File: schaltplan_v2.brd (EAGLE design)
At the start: 101 x 80 mm, 42 parts, among them T1 2N3565, T2 2N3565, T3 2N3565, T4 2N3565, T5 2N3565, T6 2N3565, T7 2N3565, T8 2N3565

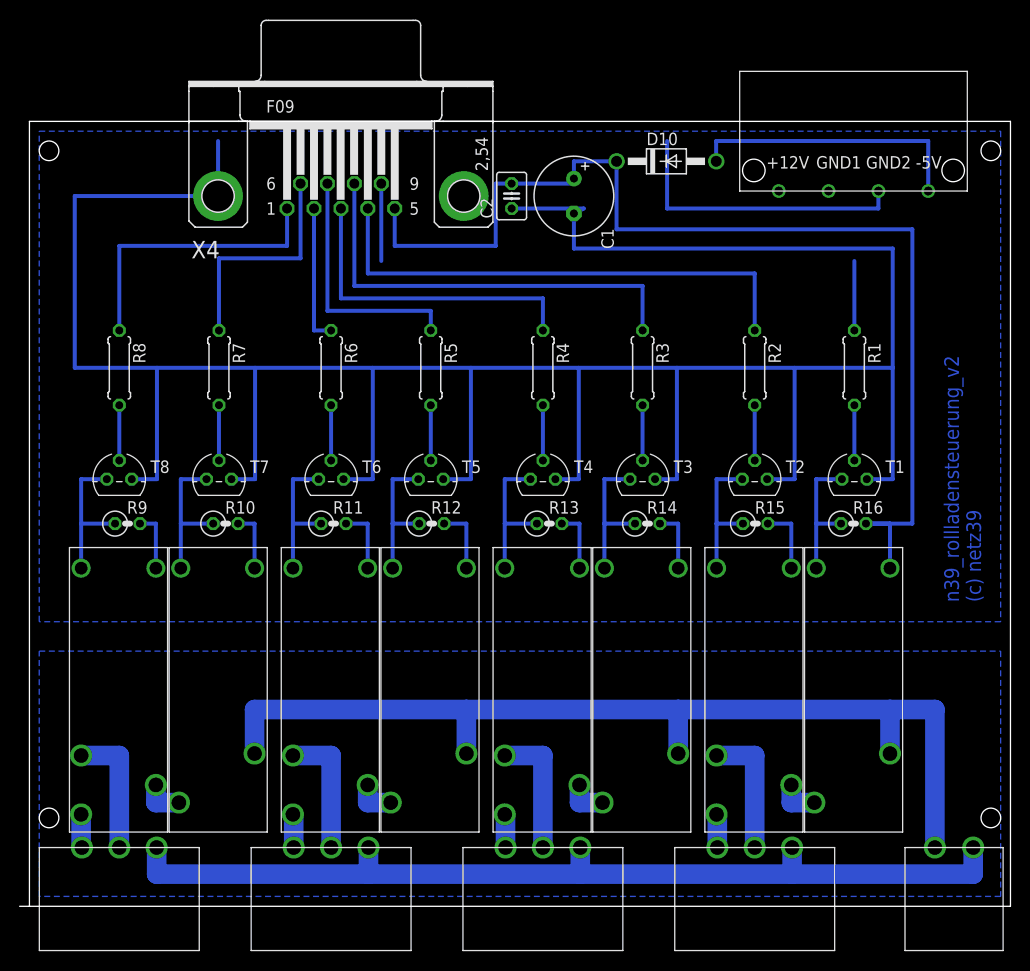
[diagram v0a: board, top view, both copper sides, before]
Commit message: minor fixes again
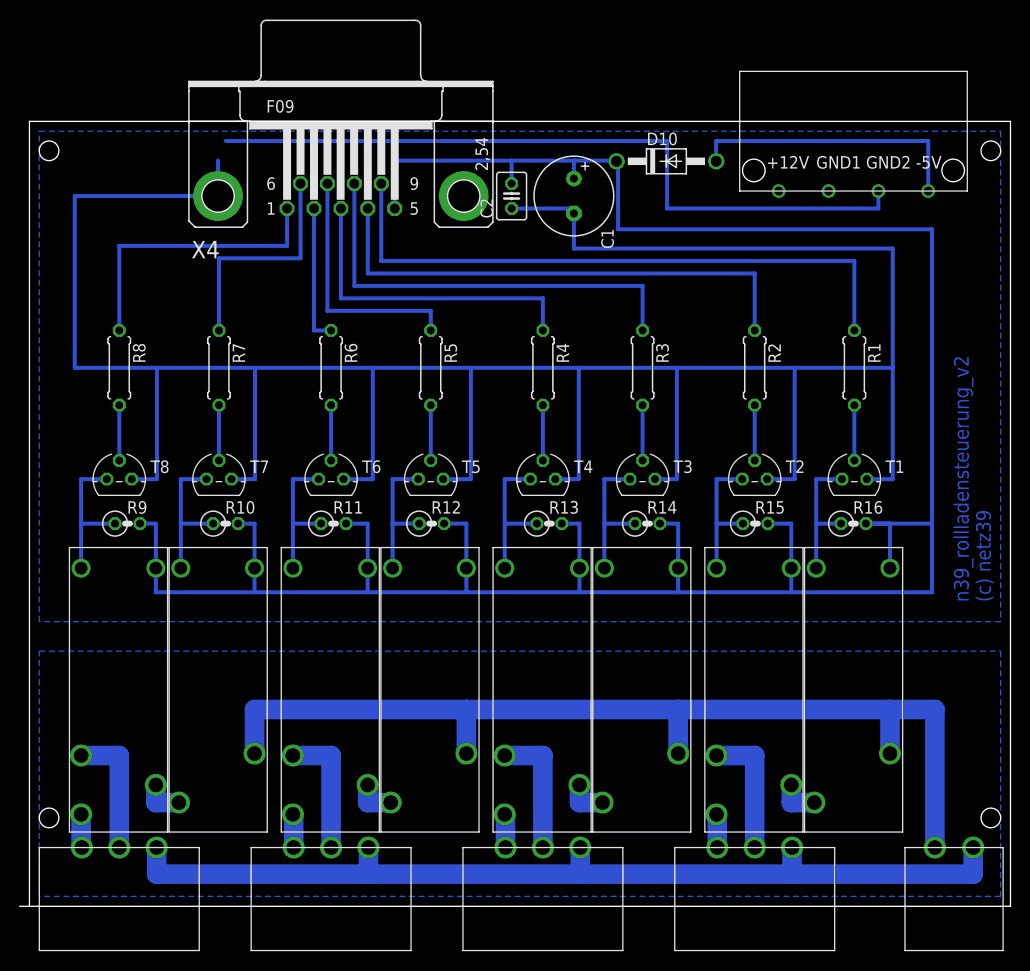
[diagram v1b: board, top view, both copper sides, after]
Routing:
- net N$24: track 159.6 -> 263.6 mm
- net N$38: track 15.0 -> 63.2 mm
- net GND: track 319.7 -> 361.0 mm
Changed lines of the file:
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@@
 <layers>
 <layer number="1" name="Top" color="4" fill="1" visible="no" active="yes"/>
-<layer number="16" name="Bottom" color="1" fill="1" visible="yes" active="yes"/>
+<layer number="16" name="Bottom" color="1" fill="1" visible="no" active="yes"/>
 <layer number="17" name="Pads" color="2" fill="1" visible="yes" active="yes"/>
 <layer number="18" name="Vias" color="2" fill="1" visible="no" active="yes"/>
-<layer number="19" name="Unrouted" color="6" fill="1" visible="yes" active="yes"/>
+<layer number="19" name="Unrouted" color="6" fill="1" visible="no" active="yes"/>
 <layer number="20" name="Dimension" color="15" fill="1" visible="yes" active="yes"/>
 <layer number="21" name="tPlace" color="7" fill="1" visible="yes" active="yes"/>
@@
 <hole x="98" y="9" drill="2"/>
 <hole x="2" y="9" drill="2"/>
-<text x="97" y="31" size="1.5" layer="16" font="vector" rot="R90">n39_rollladensteuerung_v2
+<text x="98" y="31" size="1.5" layer="16" font="vector" rot="R90">n39_rollladensteuerung_v2
 (c) netz39</text>
 </plain>
@@
 <contactref element="U$7" pad="P$2"/>
 <contactref element="U$8" pad="P$2"/>
-<wire x1="56.07" y1="39" x2="56.07" y2="34.46" width="0.4064" layer="16"/>
-<wire x1="66.13" y1="39" x2="66.13" y2="34.46" width="0.4064" layer="16"/>
-<wire x1="44.54" y1="39" x2="44.54" y2="34.46" width="0.4064" layer="16"/>
-<wire x1="34.48" y1="39" x2="34.48" y2="34.46" width="0.4064" layer="16"/>
 <wire x1="87.72" y1="39" x2="87.72" y2="34.46" width="0.4064" layer="16"/>
-<wire x1="22.95" y1="39" x2="22.95" y2="34.46" width="0.4064" layer="16"/>
-<wire x1="12.89" y1="34.46" x2="12.97" y2="34.46" width="0.4064" layer="16"/>
-<wire x1="77.66" y1="34.46" x2="77.74" y2="34.46" width="0.4064" layer="16"/>
-<wire x1="47.53" y1="73.66" x2="49.15" y2="73.66" width="0.4064" layer="16"/>
 <contactref element="X4" pad="5"/>
-<wire x1="47.53" y1="73.66" x2="47.53" y2="67.31" width="0.4064" layer="16"/>
-<wire x1="47.53" y1="67.31" x2="37.2364" y2="67.31" width="0.4064" layer="16"/>
-<wire x1="37.2364" y1="67.31" x2="37.2364" y2="71.12" width="0.4064" layer="16"/>
 <contactref element="R9" pad="2"/>
 <contactref element="R10" pad="2"/>
@@
 <contactref element="R16" pad="2"/>
 <wire x1="85.27" y1="39" x2="87.72" y2="39" width="0.4064" layer="16"/>
-<wire x1="75.27" y1="39" x2="77.66" y2="39" width="0.4064" layer="16"/>
-<wire x1="77.66" y1="39" x2="77.66" y2="34.46" width="0.4064" layer="16"/>
+<wire x1="85.27" y1="39" x2="92" y2="39" width="0.4064" layer="16"/>
+<wire x1="92" y1="39" x2="92" y2="32" width="0.4064" layer="16"/>
+<wire x1="92" y1="32" x2="77.66" y2="32" width="0.4064" layer="16"/>
+<wire x1="77.66" y1="32" x2="77.66" y2="34.46" width="0.4064" layer="16"/>
+<wire x1="66.13" y1="34.46" x2="66.13" y2="32" width="0.4064" layer="16"/>
+<wire x1="66.13" y1="32" x2="77.66" y2="32" width="0.4064" layer="16"/>
+<wire x1="56.07" y1="34.46" x2="56.07" y2="32" width="0.4064" layer="16"/>
+<wire x1="56.07" y1="32" x2="66.13" y2="32" width="0.4064" layer="16"/>
+<wire x1="44.54" y1="34.46" x2="44.54" y2="32" width="0.4064" layer="16"/>
+<wire x1="44.54" y1="32" x2="56.07" y2="32" width="0.4064" layer="16"/>
+<wire x1="34.48" y1="34.46" x2="34.48" y2="32" width="0.4064" layer="16"/>
+<wire x1="34.48" y1="32" x2="44.54" y2="32" width="0.4064" layer="16"/>
+<wire x1="22.95" y1="34.46" x2="22.95" y2="32" width="0.4064" layer="16"/>
+<wire x1="22.95" y1="32" x2="34.48" y2="32" width="0.4064" layer="16"/>
+<wire x1="12.89" y1="34.46" x2="12.89" y2="32" width="0.4064" layer="16"/>
+<wire x1="12.89" y1="32" x2="22.95" y2="32" width="0.4064" layer="16"/>
 <wire x1="11.27" y1="39" x2="12.89" y2="39" width="0.4064" layer="16"/>
 <wire x1="12.89" y1="39" x2="12.89" y2="34.46" width="0.4064" layer="16"/>
 <wire x1="21.27" y1="39" x2="22.95" y2="39" width="0.4064" layer="16"/>
+<wire x1="22.95" y1="39" x2="22.95" y2="34.46" width="0.4064" layer="16"/>
 <wire x1="32.27" y1="39" x2="34.48" y2="39" width="0.4064" layer="16"/>
+<wire x1="34.48" y1="39" x2="34.48" y2="34.46" width="0.4064" layer="16"/>
 <wire x1="42.27" y1="39" x2="44.54" y2="39" width="0.4064" layer="16"/>
+<wire x1="44.54" y1="39" x2="44.54" y2="34.46" width="0.4064" layer="16"/>
 <wire x1="54.27" y1="39" x2="56.07" y2="39" width="0.4064" layer="16"/>
+<wire x1="56.07" y1="39" x2="56.07" y2="34.46" width="0.4064" layer="16"/>
 <wire x1="64.27" y1="39" x2="66.13" y2="39" width="0.4064" layer="16"/>
-<wire x1="49.15" y1="73.66" x2="55.5" y2="73.66" width="0.4064" layer="16"/>
-<wire x1="55.5" y1="73.66" x2="55.5" y2="74.168" width="0.4064" layer="16"/>
-<wire x1="59.85" y1="75.93" x2="55.5" y2="75.93" width="0.4064" layer="16"/>
-<wire x1="55.5" y1="75.93" x2="55.5" y2="74.168" width="0.4064" layer="16"/>
-<wire x1="85.27" y1="39" x2="90" y2="39" width="0.4064" layer="16"/>
-<wire x1="90" y1="39" x2="90" y2="69" width="0.4064" layer="16"/>
-<wire x1="90" y1="69" x2="59.85" y2="69" width="0.4064" layer="16"/>
-<wire x1="59.85" y1="69" x2="59.85" y2="75.93" width="0.4064" layer="16"/>
-<wire x1="85.27" y1="39" x2="77.66" y2="39" width="0" layer="19" extent="16-16"/>
-<wire x1="66.13" y1="39" x2="75.27" y2="39" width="0" layer="19" extent="16-16"/>
-<wire x1="56.07" y1="39" x2="64.27" y2="39" width="0" layer="19" extent="16-16"/>
-<wire x1="44.54" y1="39" x2="54.27" y2="39" width="0" layer="19" extent="16-16"/>
-<wire x1="34.48" y1="39" x2="42.27" y2="39" width="0" layer="19" extent="16-16"/>
-<wire x1="22.95" y1="39" x2="32.27" y2="39" width="0" layer="19" extent="16-16"/>
-<wire x1="12.89" y1="39" x2="21.27" y2="39" width="0" layer="19" extent="16-16"/>
+<wire x1="66.13" y1="39" x2="66.13" y2="34.46" width="0.4064" layer="16"/>
+<wire x1="75.27" y1="39" x2="77.66" y2="39" width="0.4064" layer="16"/>
+<wire x1="77.66" y1="39" x2="77.66" y2="34.46" width="0.4064" layer="16"/>
+<wire x1="37.2364" y1="76" x2="49.15" y2="76" width="0.4064" layer="16"/>
+<wire x1="49.15" y1="76" x2="55.5" y2="76" width="0.4064" layer="16"/>
+<wire x1="55.5" y1="76" x2="60" y2="76" width="0.4064" layer="16"/>
+<wire x1="60" y1="75.93" x2="59.85" y2="75.93" width="0.4064" layer="16"/>
+<wire x1="55.5" y1="74.168" x2="55.5" y2="76" width="0.4064" layer="16"/>
+<wire x1="49.15" y1="73.66" x2="49.15" y2="76" width="0.4064" layer="16"/>
+<wire x1="37.2364" y1="71.12" x2="37.2364" y2="76" width="0.4064" layer="16"/>
+<wire x1="60" y1="76" x2="60" y2="75.93" width="0.4064" layer="16"/>
+<wire x1="60" y1="75.93" x2="60" y2="69" width="0.4064" layer="16"/>
+<wire x1="60" y1="69" x2="92" y2="69" width="0.4064" layer="16"/>
+<wire x1="92" y1="69" x2="92" y2="39" width="0.4064" layer="16"/>
 </signal>
 <signal name="GND">
@@
 <wire x1="86.54" y1="71.12" x2="65" y2="71.12" width="0.4064" layer="16"/>
 <wire x1="65" y1="71.12" x2="65" y2="78" width="0.4064" layer="16"/>
-<wire x1="19.2278" y1="78" x2="19.2278" y2="72.39" width="0.4064" layer="16"/>
-<wire x1="49.15" y1="71.12" x2="56.5" y2="71.12" width="0.4064" layer="16"/>
-<wire x1="56.5" y1="71.12" x2="55.5" y2="70.612" width="0.4064" layer="16"/>
+<wire x1="19.2278" y1="76" x2="19.2278" y2="72.39" width="0.4064" layer="16"/>
+<wire x1="49.15" y1="71.12" x2="55.5" y2="71.12" width="0.4064" layer="16"/>
+<wire x1="55.5" y1="71.12" x2="55.5" y2="70.612" width="0.4064" layer="16"/>
 <polygon width="0.4064" layer="16">
 <vertex x="1" y="79"/>
@@
 <wire x1="88" y1="67.04" x2="55.5" y2="67.04" width="0.4064" layer="16"/>
 <wire x1="55.5" y1="67.04" x2="55.5" y2="70.612" width="0.4064" layer="16"/>
+<wire x1="20" y1="78" x2="65" y2="78" width="0.4064" layer="16"/>
 </signal>
 <signal name="N$11">
@@
 <contactref element="X4" pad="9"/>
 <wire x1="84.09" y1="58.69" x2="84.09" y2="65.77" width="0.4064" layer="16"/>
-<wire x1="35.8648" y1="65.77" x2="35.8648" y2="73.66" width="0.4064" layer="16"/>
-<wire x1="35.8648" y1="65.77" x2="84.09" y2="65.77" width="0" layer="19" extent="16-16"/>
+<wire x1="84.09" y1="65.77" x2="35.8648" y2="65.77" width="0.4064" layer="16"/>
+<wire x1="35.8648" y1="73.66" x2="35.8648" y2="65.77" width="0.4064" layer="16"/>
 </signal>
 <signal name="GND2">
@@
 </signal>
 </signals>
+<errors>
+</errors>
 </board>
 </drawing>
